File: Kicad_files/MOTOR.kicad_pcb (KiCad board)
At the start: 2 copper layers, 113 x 53.3 mm, 4 parts, among them J1 Screw_Terminal_01x02, J2 Conn_01x08_Pin, U1 NodeMCU1.0(ESP-12E)

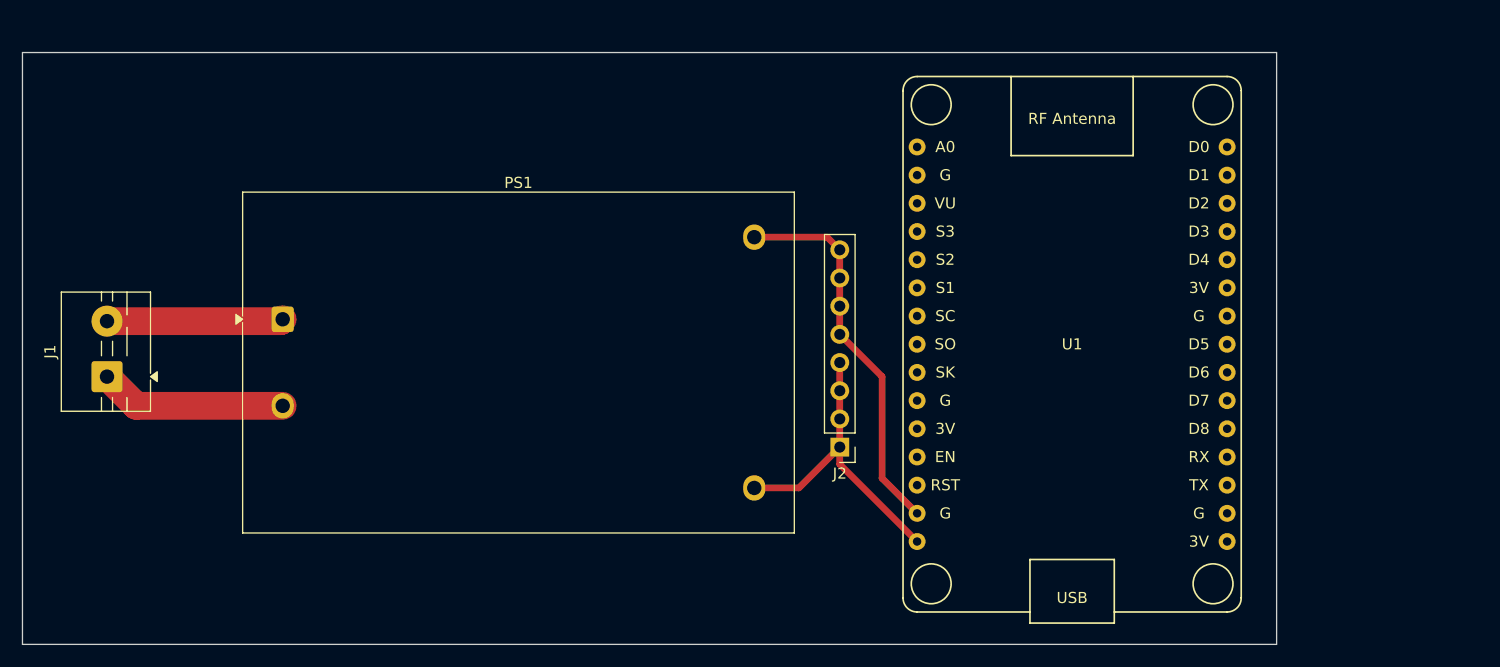
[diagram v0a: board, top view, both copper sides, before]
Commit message: feat(generated_fab_files): generated_fab_files
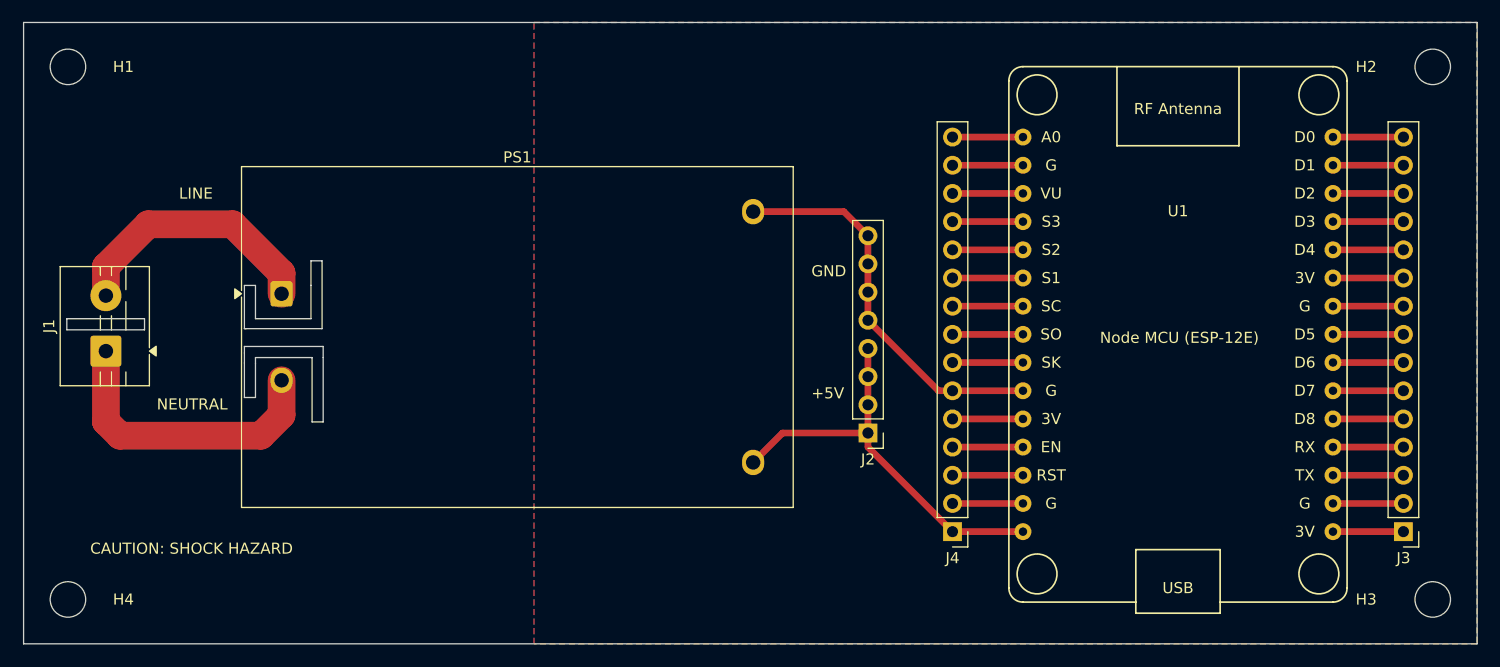
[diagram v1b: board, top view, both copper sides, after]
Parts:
- added H1: MountingHole, MountingHole:MountingHole_3.2mm_M3, F.Cu at (93.0, 94.0)
- added H2: MountingHole, MountingHole:MountingHole_3.2mm_M3, F.Cu at (216.0, 94.0)
- added H3: MountingHole, MountingHole:MountingHole_3.2mm_M3, F.Cu at (216.0, 142.0)
- added H4: MountingHole, MountingHole:MountingHole_3.2mm_M3, F.Cu at (93.0, 142.0)
- added J3: Conn_01x15_Pin, Connector_PinHeader_2.54mm:PinHeader_1x15_P2.54mm_Vertical, F.Cu at (213.4, 135.9)
- added J4: Conn_01x15_Pin, Connector_PinHeader_2.54mm:PinHeader_1x15_P2.54mm_Vertical, F.Cu at (172.7, 135.9)
- moved U1 9.58 mm to (193.0, 118.1)
- moved J2 2.84 mm to (165.1, 127.0)
- moved PS1 2.30 mm to (112.3, 114.5)
- moved J1 2.30 mm to (96.4, 119.6)
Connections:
- U1 pad 1: unconnected-(U1-A0(ADC0)-Pad1) -> /A0(ADC0)
- U1 pad 10: unconnected-(U1-GND-Pad10) -> GND
- U1 pad 11: unconnected-(U1-3.3V-Pad11) -> /3.3V
- U1 pad 12: unconnected-(U1-EN-Pad12) -> /EN
- U1 pad 13: unconnected-(U1-RST-Pad13) -> /RST
- U1 pad 16: unconnected-(U1-3.3V-Pad16) -> /3.3V
- U1 pad 17: unconnected-(U1-GND-Pad17) -> GND
- U1 pad 18: unconnected-(U1-TX(GPIO1)-Pad18) -> /TX(GPIO1)
- U1 pad 19: unconnected-(U1-RX(DPIO3)-Pad19) -> /RX(DPIO3)
- U1 pad 2: unconnected-(U1-RSV-Pad2) -> /RSV
- U1 pad 20: unconnected-(U1-D8(GPIO15)-Pad20) -> /D8(GPIO15)
- U1 pad 21: unconnected-(U1-D7(GPIO13)-Pad21) -> /D7(GPIO13)
- U1 pad 22: unconnected-(U1-D6(GPIO12)-Pad22) -> /D6(GPIO12)
- U1 pad 23: unconnected-(U1-D5(GPIO14)-Pad23) -> /D5(GPIO14)
- U1 pad 24: unconnected-(U1-GND-Pad24) -> GND
- U1 pad 25: unconnected-(U1-3.3V-Pad25) -> /3.3V
- U1 pad 26: unconnected-(U1-D4(GPIO2)-Pad26) -> /D4(GPIO2)
- U1 pad 27: unconnected-(U1-D3(GPIO0)-Pad27) -> /D3(GPIO0)
- U1 pad 28: unconnected-(U1-D2(GPIO4)-Pad28) -> /D2(GPIO4)
- U1 pad 29: unconnected-(U1-D1(GPIO5)-Pad29) -> /D1(GPIO5)
- U1 pad 3: unconnected-(U1-RSV-Pad3) -> /RSV
- U1 pad 30: unconnected-(U1-D0(GPIO16)-Pad30) -> /D0(GPIO16)
- U1 pad 4: unconnected-(U1-SD3(GPIO10)-Pad4) -> /SD3(GPIO10)
- U1 pad 5: unconnected-(U1-SD2(GPIO9)-Pad5) -> /SD2(GPIO9)
- U1 pad 6: unconnected-(U1-SD1(MOSI)-Pad6) -> /SD1(MOSI)
- U1 pad 7: unconnected-(U1-CMD(CS)-Pad7) -> /CMD(CS)
- U1 pad 8: unconnected-(U1-SDO(MISO)-Pad8) -> /SDO(MISO)
- U1 pad 9: unconnected-(U1-CLK(SCLK)-Pad9) -> /CLK(SCLK)
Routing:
- net GND: track 34.8 -> 54.7 mm
- net /3.3V: track 0.00 -> 19.1 mm
- net /RSV: track 0.00 -> 12.7 mm
- net /AC_N: track 16.9 -> 26.6 mm
- net VCC: track 28.2 -> 37.5 mm
- net /AC_L: track 15.9 -> 23.7 mm
- net /TX(GPIO1): track 0.00 -> 6.35 mm
- net /RX(DPIO3): track 0.00 -> 6.35 mm
- net /D8(GPIO15): track 0.00 -> 6.35 mm
- net /D7(GPIO13): track 0.00 -> 6.35 mm
- net /D6(GPIO12): track 0.00 -> 6.35 mm
- net /D5(GPIO14): track 0.00 -> 6.35 mm
- net /D4(GPIO2): track 0.00 -> 6.35 mm
- net /D3(GPIO0): track 0.00 -> 6.35 mm
- net /D2(GPIO4): track 0.00 -> 6.35 mm
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- added copper zone on B.Cu, net GND
- added copper zone on F.Cu, net GND
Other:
- board size 113 x 53.3 mm -> 131 x 56 mm
- board text added: "+5V"
- board text added: "CAUTION: SHOCK HAZARD"
- board text added: "GND"
- board text added: "LINE"
- board text added: "NEUTRAL"
- board text added: "Node MCU (ESP-12E)"
